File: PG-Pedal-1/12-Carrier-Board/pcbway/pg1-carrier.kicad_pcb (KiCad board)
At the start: 2 copper layers, 111 x 58.2 mm, 102 parts, among them J1 in, J10 seed3 + 9v, J19 pg-hp, J2 out, J20 pg-line, J21 expansion, J22 fx loop, U1 AMS1117-5.0, U10 TPA6139A2, U11 OPA1652, U12 OPA1652, U2 LP2985-33, U3 B0505S-1WR3, U4 ISO7741, U5 ISO1540, U7 LP2985-33, U8 OPA1652, U9 TLV320AIC3204

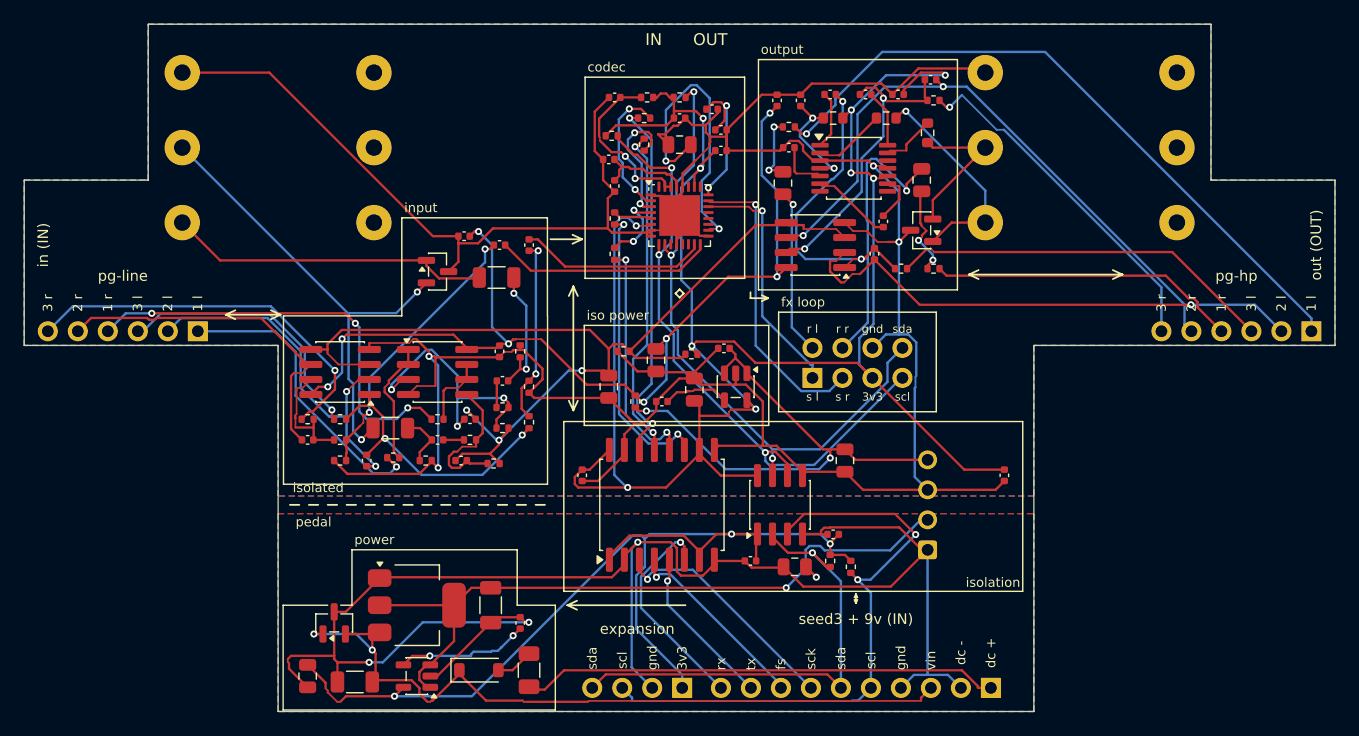
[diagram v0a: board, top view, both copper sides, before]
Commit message: Carrier: ~$50 build (TLV9062, XC6206 basic parts, through-hole parts hand-soldered)
Co-Authored-By: Claude Opus 5.5 <noreply@anthropic.com>
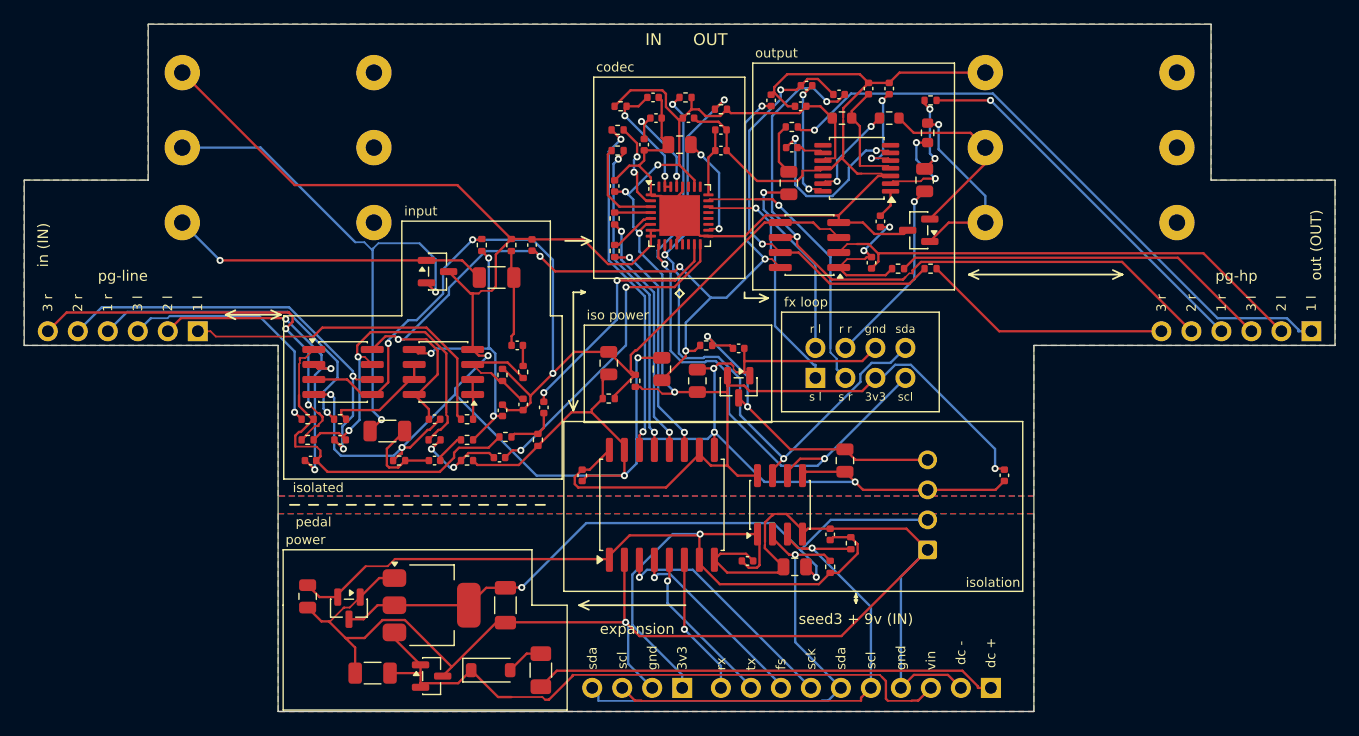
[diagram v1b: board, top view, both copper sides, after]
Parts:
- removed C13, C5: 10nF, C_0402_1005Metric
- U11, U12, U8: value OPA1652 -> TLV9062
- U2, U7: value LP2985-33 -> XC6206P332MR; footprint SOT-23-5 -> SOT-23
- moved R43 18.5 mm to (83.2, 48.5), turned to 90 degrees
- moved C42 18.0 mm to (84.8, 66.5)
- moved R61 14.3 mm to (121.2, 36.2)
- moved R62 14.3 mm to (121.2, 50.5)
- moved C32 13.8 mm to (88.5, 62.2)
- moved C51 11.6 mm to (117.0, 46.5), turned to 90 degrees
- moved R45 10.8 mm to (82.0, 66.8), turned to 0 degrees
- moved C70 9.96 mm to (109.5, 40.2), turned to 180 degrees
- moved C71 9.86 mm to (117.8, 35.2), turned to -90 degrees
- moved C23 9.49 mm to (94.5, 43.5), turned to 90 degrees
- moved D2 9.40 mm to (79.0, 85.0), turned to 0 degrees
- moved R31 9.03 mm to (85.8, 48.5)
- moved C72 8.31 mm to (110.2, 36.8)
- moved R46 8.25 mm to (71.2, 63.2)
- moved U2 8.13 mm to (72.0, 79.2), turned to -90 degrees
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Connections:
- U2 pad 1: +5V -> GND
- U2 pad 2: GND -> +3V3
- U7 pad 1: ISO5V_RAW -> IGND
- U7 pad 2: IGND -> ISO3V3
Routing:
- net ISO3V3: track 177.5 -> 127.8 mm, vias 10 -> 5
- net IGND: track 290.6 -> 314.6 mm, vias 4 -> 8
- net IN_G_R: track 9.96 -> 30.0 mm, vias 0 -> 2
- net IN_E_R: track 23.9 -> 7.69 mm
- net REF: track 24.9 -> 9.07 mm
- net ISO5V_RAW: track 42.5 -> 28.3 mm
- net OUT_G_L: track 26.7 -> 12.8 mm
- net IN_C_R: track 12.3 -> 24.7 mm, vias 0 -> 3
- net IN_C_L: track 22.1 -> 10.4 mm, vias 3 -> 0
- net IN_E_L: track 15.6 -> 4.31 mm, vias 2 -> 0
- net PBYP: track 11.2 -> 0.00 mm, vias 2 -> 0
- net OUT_G_R: track 25.6 -> 35.7 mm
- net CIN2_R: track 18.6 -> 27.7 mm, vias 0 -> 2
- net GIN_A_R: track 36.7 -> 27.6 mm, vias 3 -> 1
- net HP_CN: track 6.89 -> 15.8 mm, vias 0 -> 2
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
